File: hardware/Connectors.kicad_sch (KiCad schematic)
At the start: 9 parts, among them J1 Harw_Conn_1x2, J10 USB_B_Mini, J14 Conn_01x05, J16 Harw_Conn_2x13, J2 Harw_Conn_1x2, J3 Harw_Conn_1x2, J8 Harw_Conn_1x4

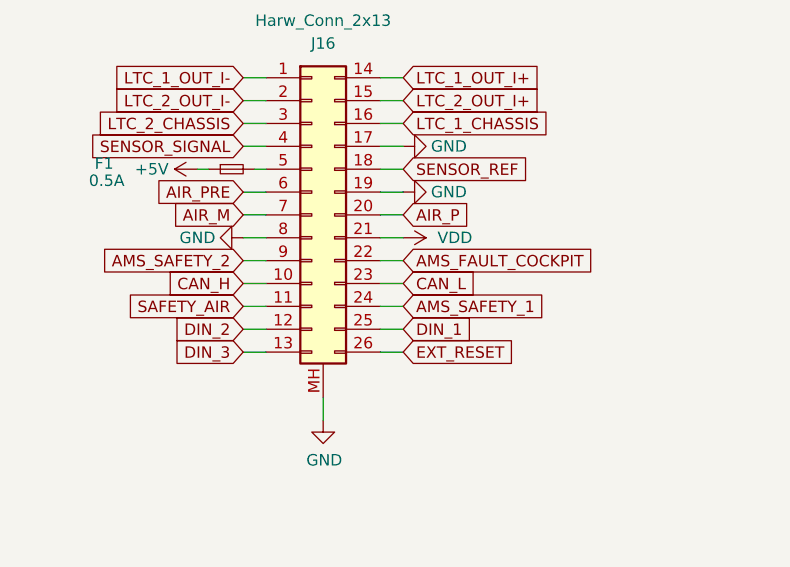
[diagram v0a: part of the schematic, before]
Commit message: finished board design
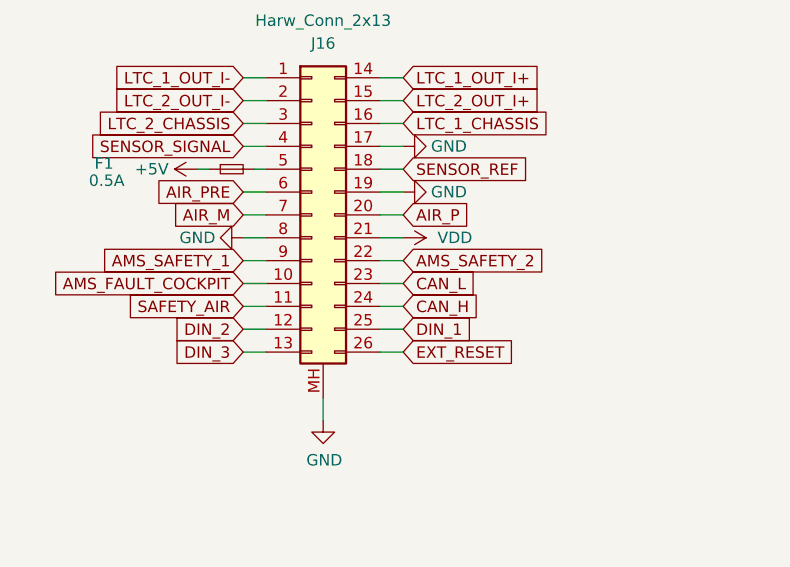
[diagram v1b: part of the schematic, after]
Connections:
- net AMS_FAULT_COCKPIT: now also J16.10; no longer J16.22
- net AMS_SAFETY_1: now also J16.9; no longer J16.24
- net AMS_SAFETY_2: now also J16.22; no longer J16.9
- net CAN_H: now also J16.24; no longer J16.10
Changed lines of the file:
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@@
     (stroke (width 0) (type default) (color 0 0 0 0))
   )
-  (wire (pts (xy 84.455 121.92) (xy 81.915 121.92))
+  (wire (pts (xy 66.675 116.84) (xy 69.215 116.84))
     (stroke (width 0) (type default) (color 0 0 0 0))
   )
@@
     (stroke (width 0) (type default) (color 0 0 0 0))
   )
+  (wire (pts (xy 84.455 121.92) (xy 81.915 121.92))
+    (stroke (width 0) (type default) (color 0 0 0 0))
+  )
+  (wire (pts (xy 240.665 63.5) (xy 240.665 64.77))
+    (stroke (width 0) (type default) (color 0 0 0 0))
+  )
+  (wire (pts (xy 250.825 46.99) (xy 250.825 43.18))
+    (stroke (width 0) (type default) (color 0 0 0 0))
+  )
+  (wire (pts (xy 180.975 137.16) (xy 178.435 137.16))
+    (stroke (width 0) (type default) (color 0 0 0 0))
+  )
+  (wire (pts (xy 250.19 111.76) (xy 250.19 113.03))
+    (stroke (width 0) (type default) (color 0 0 0 0))
+  )
+  (wire (pts (xy 179.705 134.62) (xy 179.705 132.08))
+    (stroke (width 0) (type default) (color 0 0 0 0))
+  )
+  (wire (pts (xy 240.665 63.5) (xy 241.935 63.5))
+    (stroke (width 0) (type default) (color 0 0 0 0))
+  )
+  (wire (pts (xy 66.675 104.14) (xy 69.215 104.14))
+    (stroke (width 0) (type default) (color 0 0 0 0))
+  )
+  (wire (pts (xy 69.215 121.92) (xy 66.675 121.92))
+    (stroke (width 0) (type default) (color 0 0 0 0))
+  )
+  (wire (pts (xy 172.72 81.915) (xy 175.26 81.915))
+    (stroke (width 0) (type default) (color 0 0 0 0))
+  )
+  (wire (pts (xy 188.595 47.625) (xy 186.055 47.625))
+    (stroke (width 0) (type default) (color 0 0 0 0))
+  )
+  (wire (pts (xy 249.555 46.99) (xy 250.825 46.99))
+    (stroke (width 0) (type default) (color 0 0 0 0))
+  )
+  (wire (pts (xy 248.92 106.045) (xy 251.46 106.045))
+    (stroke (width 0) (type default) (color 0 0 0 0))
+  )
+  (wire (pts (xy 184.785 48.895) (xy 186.055 48.895))
+    (stroke (width 0) (type default) (color 0 0 0 0))
+  )
   (wire (pts (xy 66.675 119.38) (xy 69.215 119.38))
-    (stroke (width 0) (type default) (color 0 0 0 0))
-  )
-  (wire (pts (xy 240.665 63.5) (xy 240.665 64.77))
-    (stroke (width 0) (type default) (color 0 0 0 0))
-  )
-  (wire (pts (xy 250.825 46.99) (xy 250.825 43.18))
-    (stroke (width 0) (type default) (color 0 0 0 0))
-  )
-  (wire (pts (xy 180.975 137.16) (xy 178.435 137.16))
-    (stroke (width 0) (type default) (color 0 0 0 0))
-  )
-  (wire (pts (xy 250.19 111.76) (xy 250.19 113.03))
-    (stroke (width 0) (type default) (color 0 0 0 0))
-  )
-  (wire (pts (xy 179.705 134.62) (xy 179.705 132.08))
-    (stroke (width 0) (type default) (color 0 0 0 0))
-  )
-  (wire (pts (xy 240.665 63.5) (xy 241.935 63.5))
-    (stroke (width 0) (type default) (color 0 0 0 0))
-  )
-  (wire (pts (xy 66.675 104.14) (xy 69.215 104.14))
-    (stroke (width 0) (type default) (color 0 0 0 0))
-  )
-  (wire (pts (xy 69.215 121.92) (xy 66.675 121.92))
-    (stroke (width 0) (type default) (color 0 0 0 0))
-  )
-  (wire (pts (xy 172.72 81.915) (xy 175.26 81.915))
-    (stroke (width 0) (type default) (color 0 0 0 0))
-  )
-  (wire (pts (xy 188.595 47.625) (xy 186.055 47.625))
-    (stroke (width 0) (type default) (color 0 0 0 0))
-  )
-  (wire (pts (xy 249.555 46.99) (xy 250.825 46.99))
-    (stroke (width 0) (type default) (color 0 0 0 0))
-  )
-  (wire (pts (xy 248.92 106.045) (xy 251.46 106.045))
-    (stroke (width 0) (type default) (color 0 0 0 0))
-  )
-  (wire (pts (xy 184.785 48.895) (xy 186.055 48.895))
-    (stroke (width 0) (type default) (color 0 0 0 0))
-  )
-  (wire (pts (xy 84.455 116.84) (xy 81.915 116.84))
     (stroke (width 0) (type default) (color 0 0 0 0))
   )
@@
     (stroke (width 0) (type default) (color 0 0 0 0))
   )
-  (wire (pts (xy 69.215 116.84) (xy 66.675 116.84))
+  (wire (pts (xy 81.915 116.84) (xy 84.455 116.84))
     (stroke (width 0) (type default) (color 0 0 0 0))
   )
@@
     )
   )
-  (global_label "CAN_H" (shape input) (at 66.675 119.38 180) (fields_autoplaced)
-    (effects (font (size 1.27 1.27)) (justify right))
-    (property "Intersheet References" "${INTERSHEET_REFS}" (id 0) (at 58.3637 119.4594 0)
-      (effects (font (size 1.27 1.27)) (justify right) hide)
+  (global_label "CAN_H" (shape input) (at 84.455 121.92 0) (fields_autoplaced)
+    (effects (font (size 1.27 1.27)) (justify left))
+    (property "Intersheet References" "${INTERSHEET_REFS}" (id 0) (at 92.7663 121.8406 0)
+      (effects (font (size 1.27 1.27)) (justify left) hide)
     )
   )
@@
     )
   )
-  (global_label "AMS_FAULT_COCKPIT" (shape input) (at 84.455 116.84 0) (fields_autoplaced)
-    (effects (font (size 1.27 1.27)) (justify left))
-    (property "Intersheet References" "${INTERSHEET_REFS}" (id 0) (at 105.9502 116.7606 0)
-      (effects (font (size 1.27 1.27)) (justify left) hide)
+  (global_label "AMS_FAULT_COCKPIT" (shape input) (at 66.675 119.38 180) (fields_autoplaced)
+    (effects (font (size 1.27 1.27)) (justify right))
+    (property "Intersheet References" "${INTERSHEET_REFS}" (id 0) (at 45.1798 119.4594 0)
+      (effects (font (size 1.27 1.27)) (justify right) hide)
     )
   )
@@
     )
   )
-  (global_label "AMS_SAFETY_2" (shape input) (at 66.675 116.84 180) (fields_autoplaced)
+  (global_label "AMS_SAFETY_2" (shape input) (at 84.455 116.84 0) (fields_autoplaced)
+    (effects (font (size 1.27 1.27)) (justify left))
+    (property "Intersheet References" "${INTERSHEET_REFS}" (id 0) (at 100.2654 116.7606 0)
+      (effects (font (size 1.27 1.27)) (justify left) hide)
+    )
+  )
+  (global_label "SWDIO" (shape input) (at 178.435 142.24 180) (fields_autoplaced)
+    (effects (font (size 1.27 1.27)) (justify right))
+    (property "Intersheet References" "${INTERSHEET_REFS}" (id 0) (at 170.2446 142.1606 0)
+      (effects (font (size 1.27 1.27)) (justify right) hide)
+    )
+  )
+  (global_label "AIR_M" (shape input) (at 66.675 111.76 180) (fields_autoplaced)
+    (effects (font (size 1.27 1.27)) (justify right))
+    (property "Intersheet References" "${INTERSHEET_REFS}" (id 0) (at 58.9684 111.8394 0)
+      (effects (font (size 1.27 1.27)) (justify right) hide)
+    )
+  )
+  (global_label "AMS_SAFETY_1" (shape input) (at 66.675 116.84 180) (fields_autoplaced)
     (effects (font (size 1.27 1.27)) (justify right))
     (property "Intersheet References" "${INTERSHEET_REFS}" (id 0) (at 50.8646 116.9194 0)
@@
     )
   )
-  (global_label "SWDIO" (shape input) (at 178.435 142.24 180) (fields_autoplaced)
-    (effects (font (size 1.27 1.27)) (justify right))
-    (property "Intersheet References" "${INTERSHEET_REFS}" (id 0) (at 170.2446 142.1606 0)
-      (effects (font (size 1.27 1.27)) (justify right) hide)
-    )
-  )
-  (global_label "AIR_M" (shape input) (at 66.675 111.76 180) (fields_autoplaced)
-    (effects (font (size 1.27 1.27)) (justify right))
-    (property "Intersheet References" "${INTERSHEET_REFS}" (id 0) (at 58.9684 111.8394 0)
-      (effects (font (size 1.27 1.27)) (justify right) hide)
-    )
-  )
-  (global_label "AMS_SAFETY_1" (shape input) (at 84.455 121.92 0) (fields_autoplaced)
-    (effects (font (size 1.27 1.27)) (justify left))
-    (property "Intersheet References" "${INTERSHEET_REFS}" (id 0) (at 100.2654 121.8406 0)
-      (effects (font (size 1.27 1.27)) (justify left) hide)
-    )
-  )

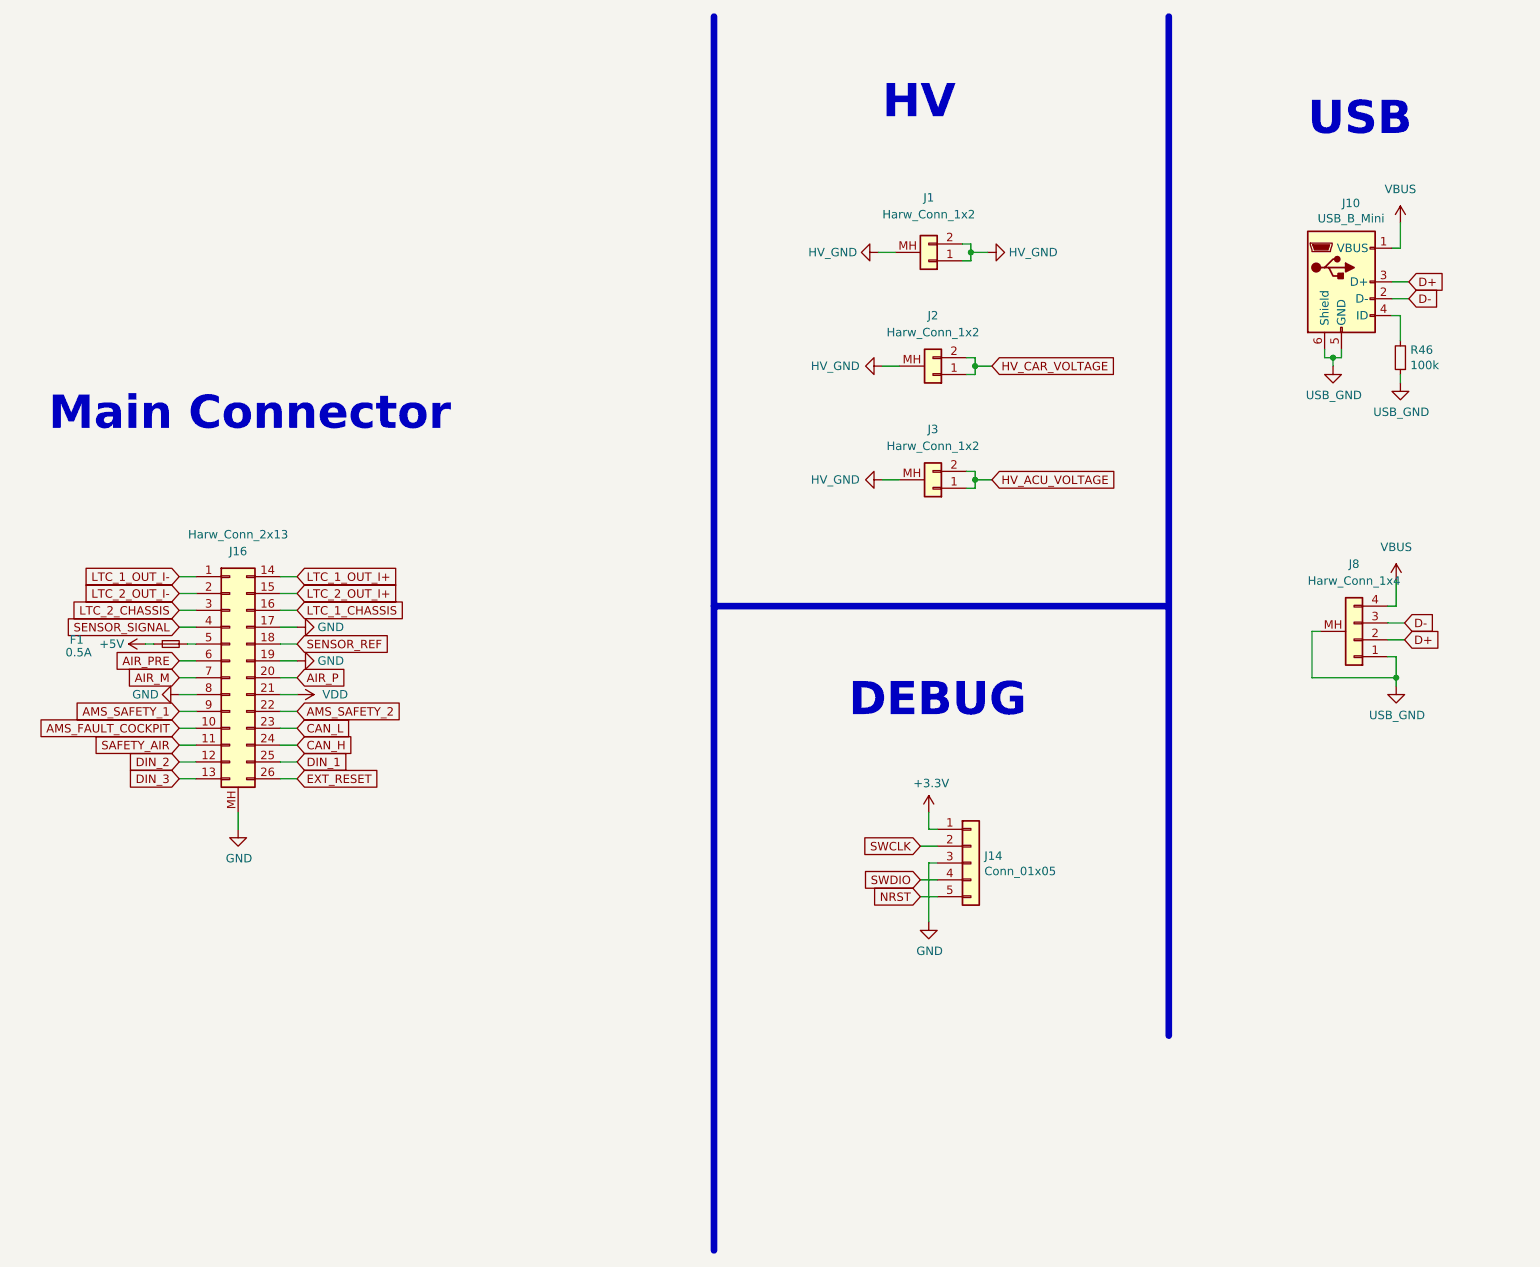
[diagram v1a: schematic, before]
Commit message: schematic override, just cuz
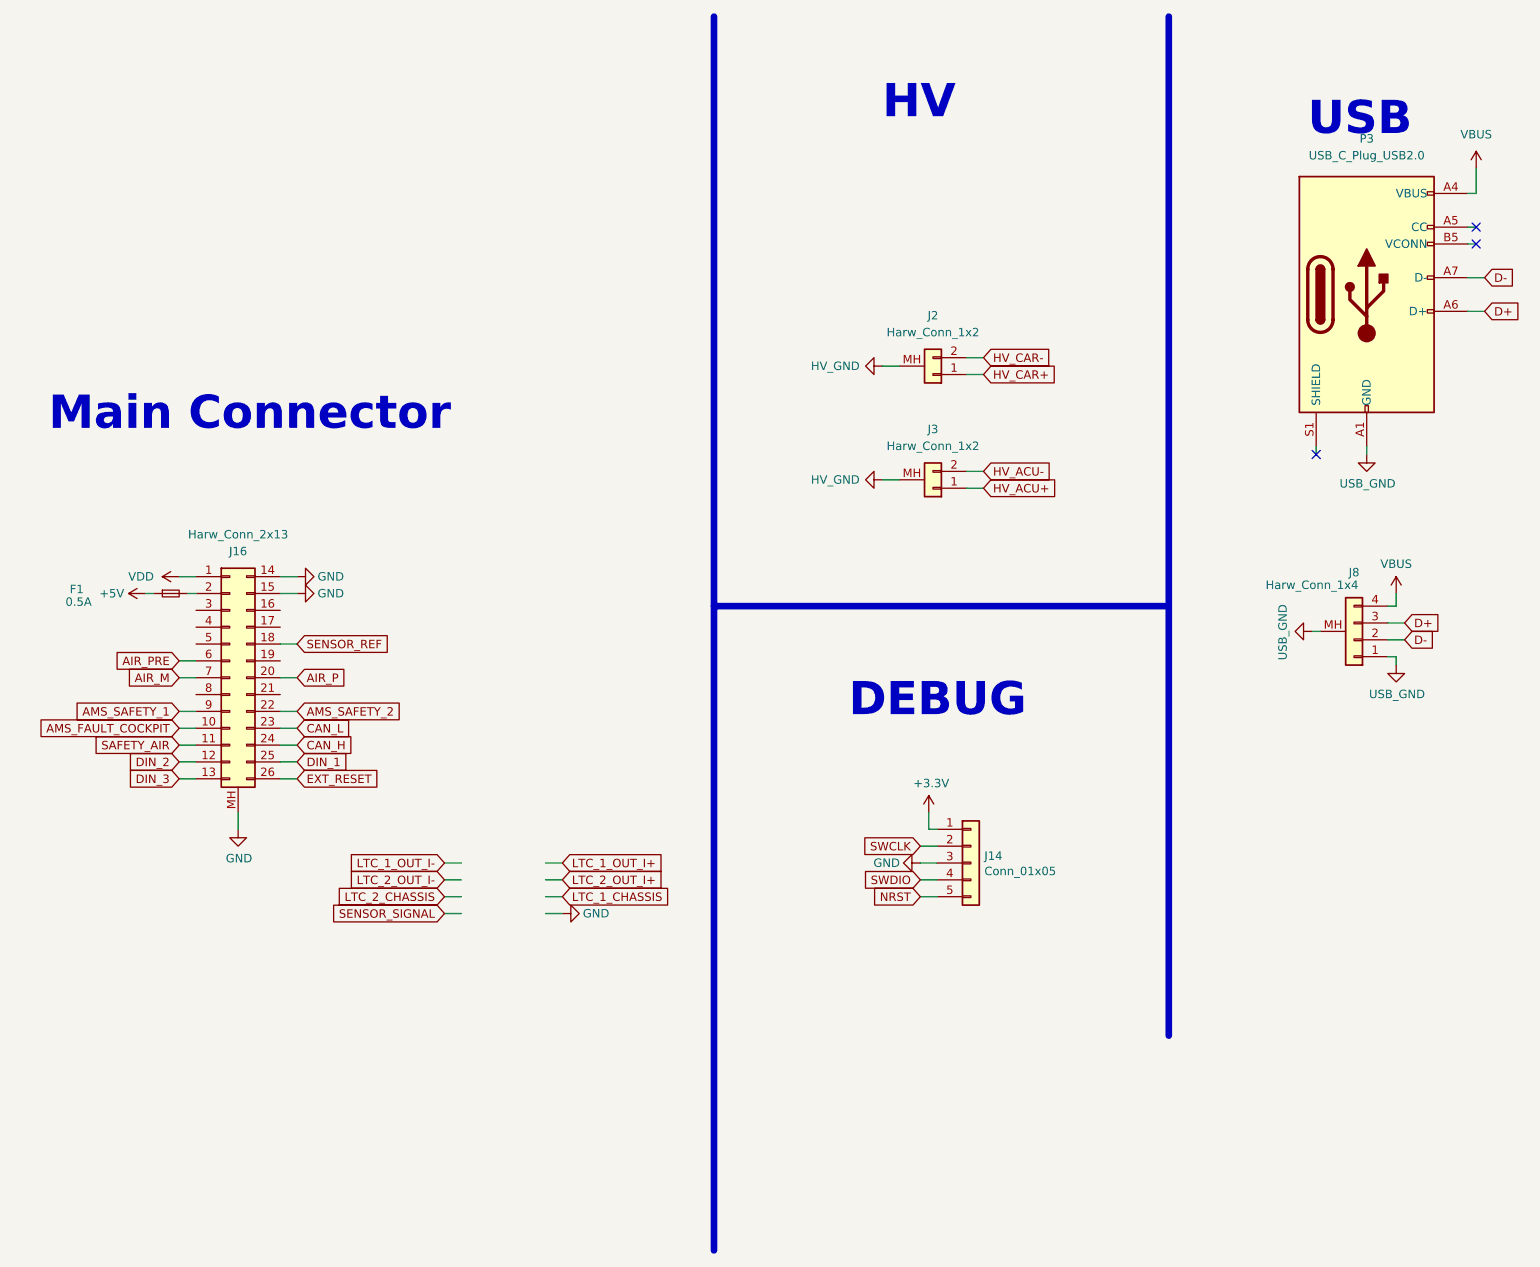
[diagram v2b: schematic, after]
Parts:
- removed J1: Harw_Conn_1x2, M808420245, symbol Harwin 2 pin 90 deg:Harw_Conn_1x2
- removed J10: USB_B_Mini, Connector_USB:USB_Mini-B_Lumberg_2486_01_Horizontal, symbol Connector:USB_B_Mini
- removed R46: 100k, Resistor_SMD:R_0603_1608Metric, symbol Device:R_Small
- added P3: USB_C_Plug_USB2.0, Connector_USB:USB_C_Receptacle_HRO_TYPE-C-31-M-12, symbol Connector:USB_C_Plug_USB2.0
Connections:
- net D+: now also J8.3, P3.A6 (D+); no longer J8.2
- net D-: now also J8.2, P3.A7 (D-); no longer J8.3
- net GND: now also J16.14, J16.15; no longer J16.17, J16.19, J16.8
- net LTC_1_CHASSIS: no longer J16.16
- net LTC_1_OUT_I+: no longer J16.14
- net LTC_1_OUT_I-: no longer J16.1
- net LTC_2_CHASSIS: no longer J16.3
- net LTC_2_OUT_I+: no longer J16.15
- net LTC_2_OUT_I-: no longer J16.2
- net SENSOR_SIGNAL: no longer J16.4
- net USB_GND: now also P3.A1 (GND), P3.A12 (GND), P3.B1 (GND), P3.B12 (GND)
- net VBUS: now also P3.A4 (VBUS), P3.A9 (VBUS), P3.B4 (VBUS), P3.B9 (VBUS)
- net VDD: now also J16.1; no longer J16.21
- net at F1.2: now also J16.2; no longer J16.5
- net HV_ACU_VOLTAGE renamed HV_ACU+
- net HV_ACU+: no longer J3.2
- net HV_CAR_VOLTAGE renamed HV_CAR+
- net HV_CAR+: no longer J2.2
- new net HV_ACU-: J3.2
- new net HV_CAR-: J2.2
- no-connect marks 0 -> 3
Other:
- moved on the sheet: F1
